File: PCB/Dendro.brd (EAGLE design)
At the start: 74.9 x 39.4 mm, 5 parts

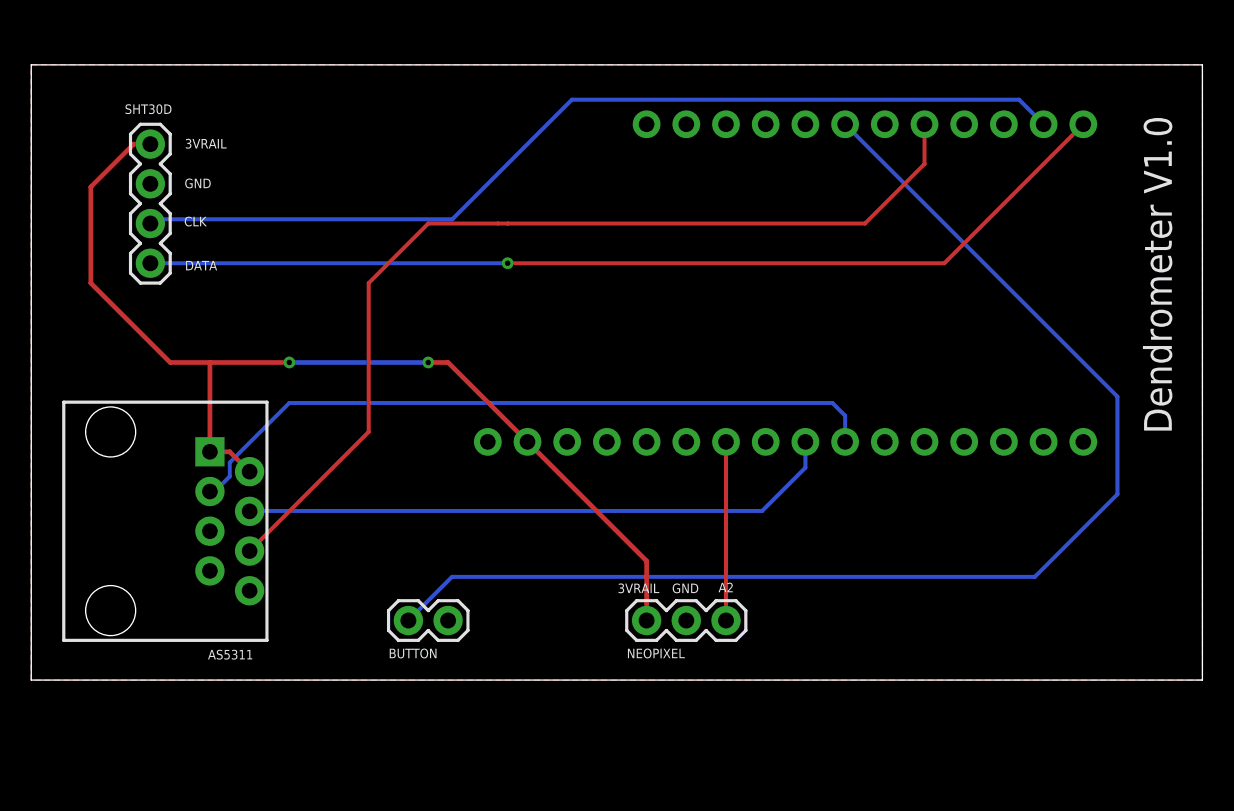
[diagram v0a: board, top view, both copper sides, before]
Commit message: Dendro PCB V1.1
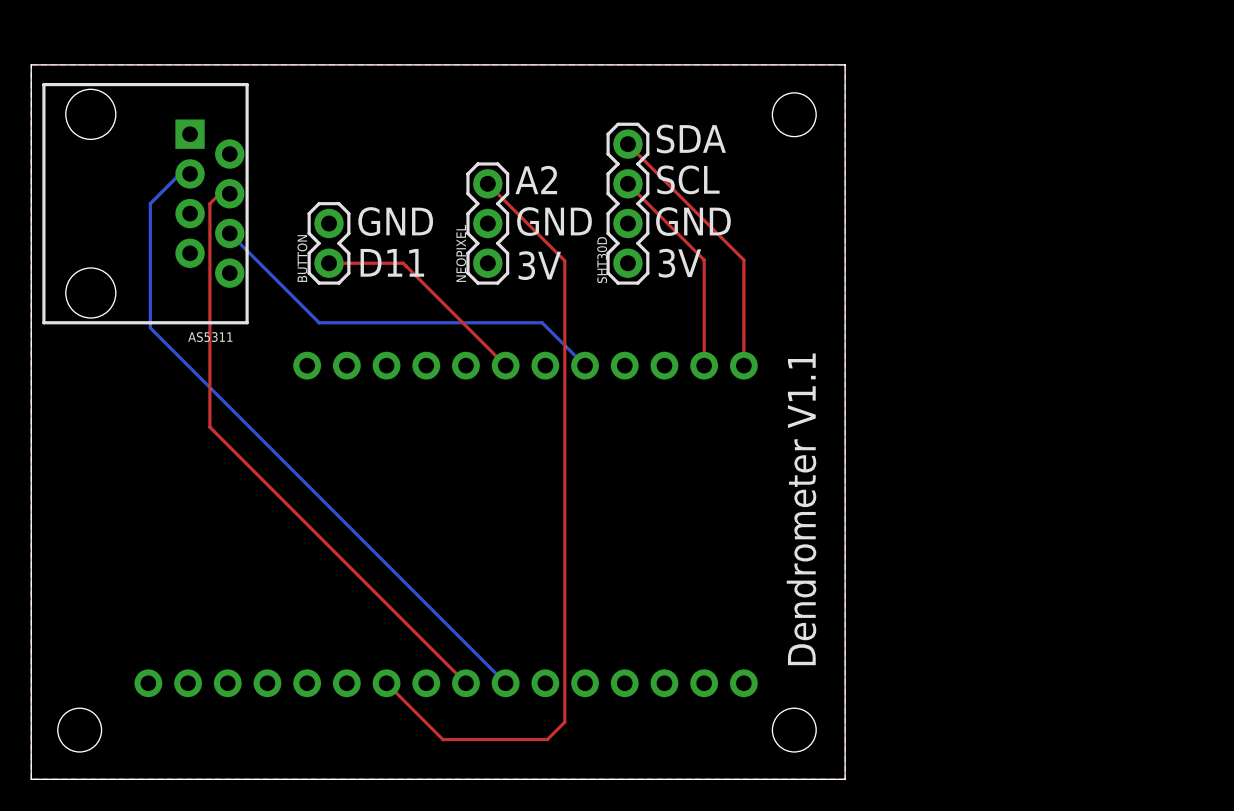
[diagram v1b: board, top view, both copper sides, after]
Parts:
- NEOPIXEL: value 455-1750-1-ND -> (none)
- moved SHT30D 31.5 mm to (38.2, 26.7), turned to 90 degrees
- moved MS1 26.6 mm to (1.14, -1.47)
- moved NEOPIXEL 25.0 mm to (29.2, 26.7), turned to 90 degrees
- moved BUTTON 23.4 mm to (19.1, 26.7), turned to 90 degrees
- moved AS5311 20.4 mm to (3.81, 30.5)
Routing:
- net 3VRAIL: track 66.6 -> 0.00 mm, vias 2 -> 0
- net D11: track 79.6 -> 14.0 mm
- net SCL: track 61.1 -> 13.7 mm
- net SDA: track 63.4 -> 17.2 mm, vias 1 -> 0
- net A2: track 11.4 -> 49.8 mm
- net CSN: track 61.6 -> 26.2 mm
- net SCLK: track 45.5 -> 43.4 mm
- net DO: track 38.4 -> 39.0 mm
- added copper zone on layer 16, net 3VRAIL
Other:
- board size 74.9 x 39.4 mm -> 52.1 x 45.7 mm
- board text added: "3V"
- board text added: "D11"
- board text added: "Dendrometer V1.1"
- board text added: "SCL"
- board text added: "SDA"
- board text removed: "3VRAIL"
- board text removed: "CLK"
- board text removed: "DATA"
- board text removed: "Dendrometer V1.0"
